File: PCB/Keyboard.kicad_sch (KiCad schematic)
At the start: 0 parts

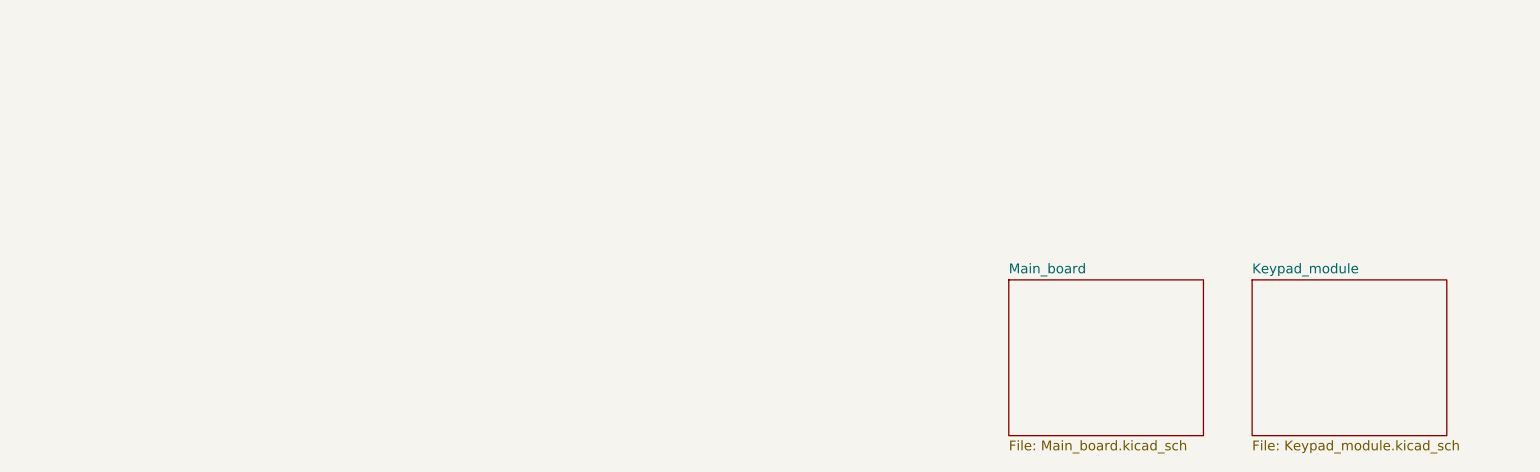
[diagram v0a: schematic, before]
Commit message: Update: Schematic and mainboard PCB
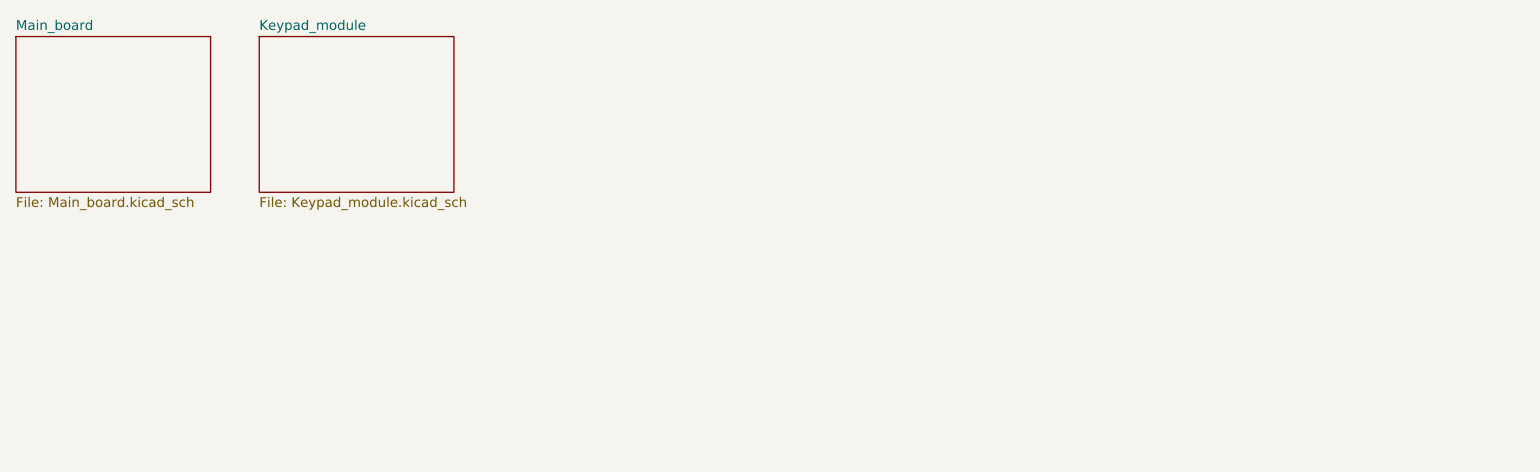
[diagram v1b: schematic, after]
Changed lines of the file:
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@@
 	(paper "A4")
 	(sheet
-		(at 214.63 76.2)
+		(at 85.09 44.45)
 		(size 25.4 20.32)
 		(exclude_from_sim no)
@@
 		)
 		(property "Sheetname" "Keypad_module"
-			(at 214.63 75.4884 0)
+			(at 85.09 43.7384 0)
 			(effects
 				(font
@@
 		)
 		(property "Sheetfile" "Keypad_module.kicad_sch"
-			(at 214.63 97.1046 0)
+			(at 85.09 65.3546 0)
 			(effects
 				(font
@@
 			(project "Keyboard"
 				(path "/fa4d5580-8795-4b64-903a-bec98e134c5c"
-					(page "3")
+					(page "4")
 				)
 			)
@@
 	)
 	(sheet
-		(at 182.88 76.2)
+		(at 53.34 44.45)
 		(size 25.4 20.32)
 		(exclude_from_sim no)
@@
 		)
 		(property "Sheetname" "Main_board"
-			(at 182.88 75.4884 0)
+			(at 53.34 43.7384 0)
 			(effects
 				(font
@@
 		)
 		(property "Sheetfile" "Main_board.kicad_sch"
-			(at 182.88 97.1046 0)
+			(at 53.34 65.3546 0)
 			(effects
 				(font
